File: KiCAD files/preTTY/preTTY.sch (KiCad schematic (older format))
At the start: 27 parts, among them J1 Power Bus, J2 Signal Buss, J3 TTL/RS232, J4 PORT0 TTL, J5 PORT1 TTL/RS232, J6 DB9, U1 74LS07, U2 ATmega328P-PU, U3 MAX232, Y1 16MHz

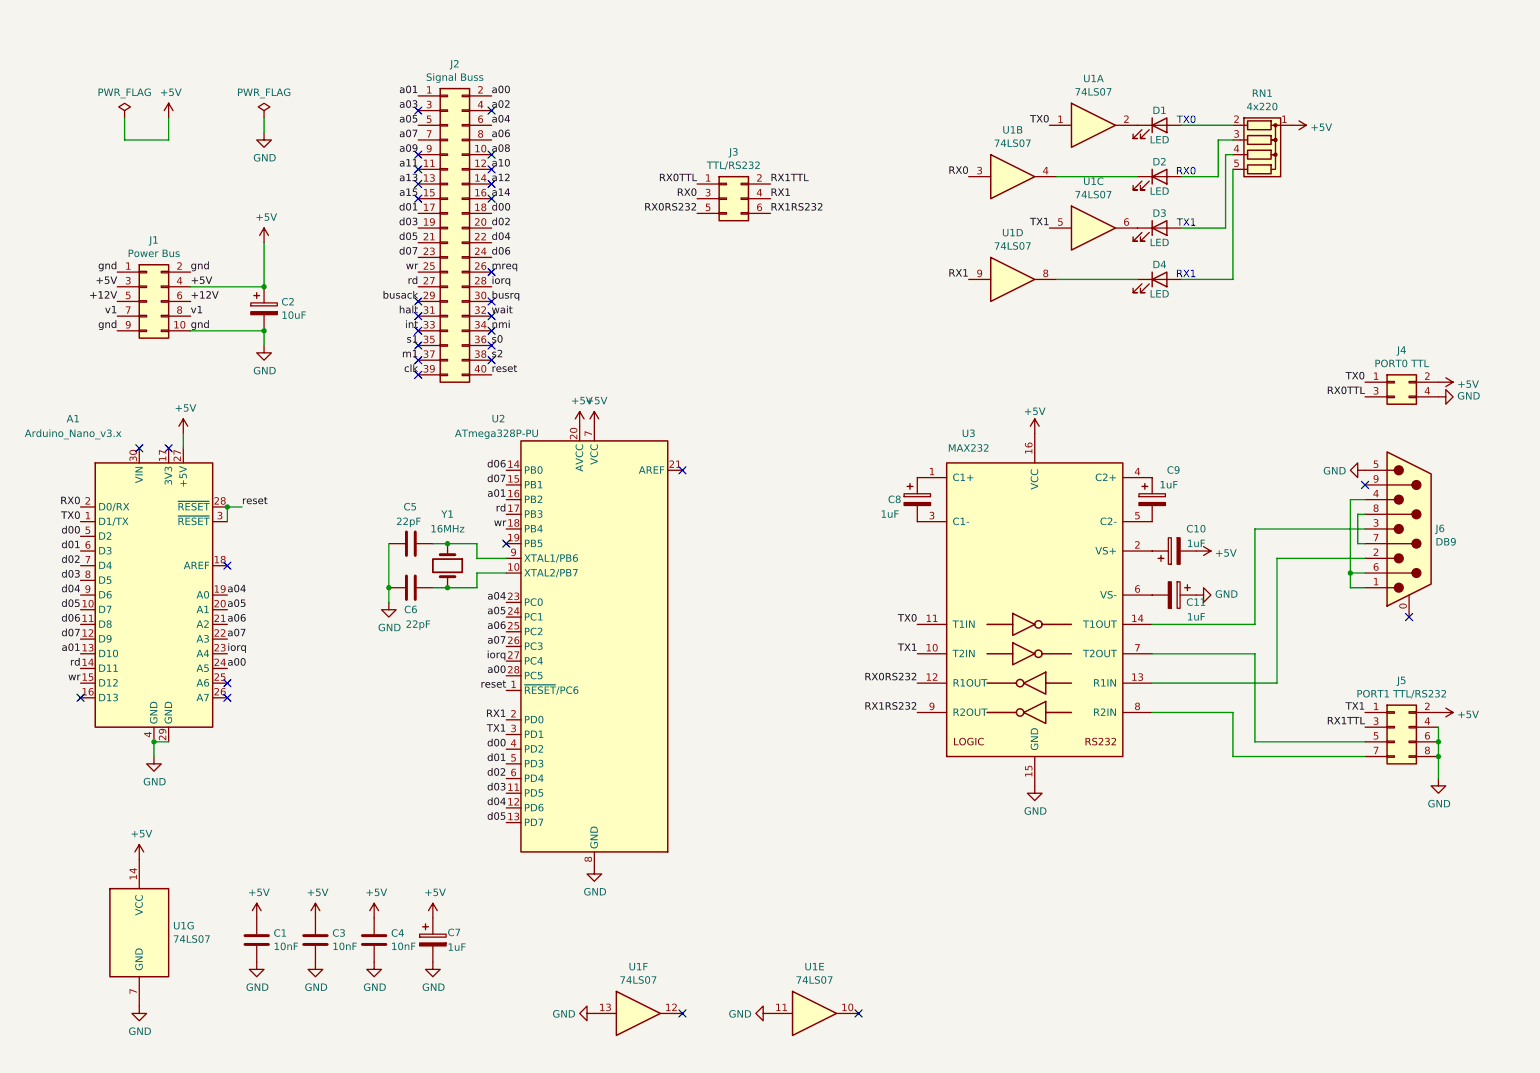
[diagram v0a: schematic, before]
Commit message: office
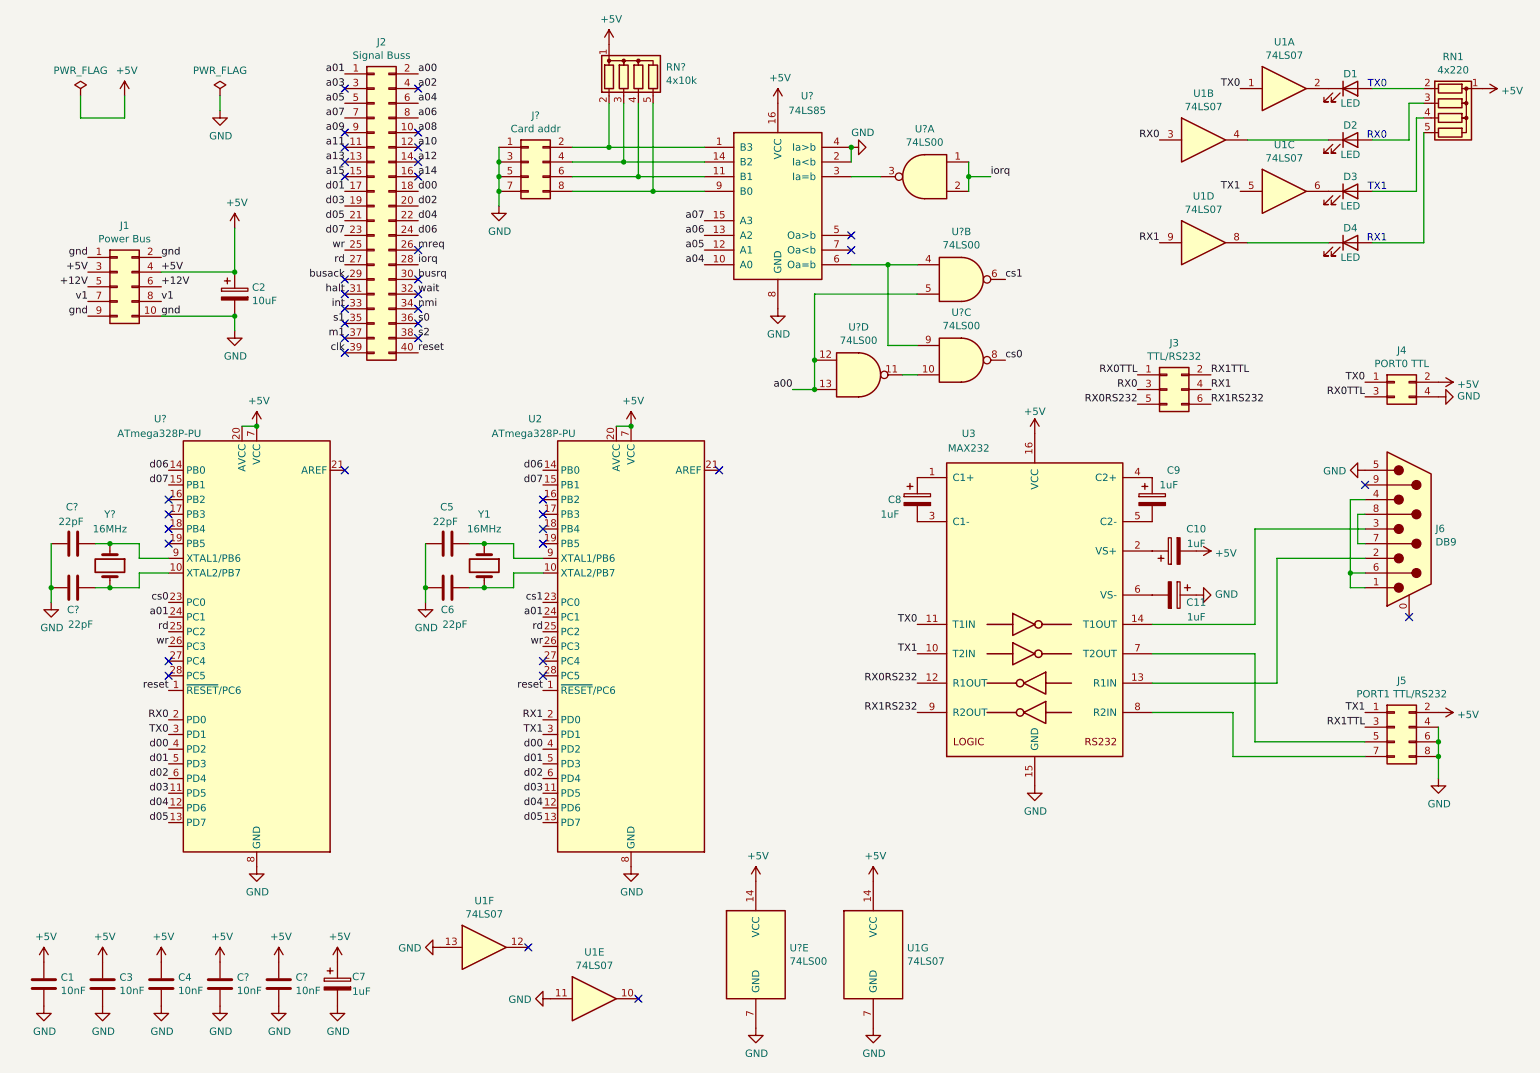
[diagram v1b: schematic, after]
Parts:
- removed A1: Arduino_Nano_v3.x, Module:Arduino_Nano, symbol preTTY-rescue:Arduino_Nano_v3.x-MCU_Module-USARTv2-rescue
- added C? (x2): 22pF, symbol Device:C
- added C? (x2): 10nF, symbol Device:C
- added J?: Card addr, symbol Connector_Generic:Conn_02x04_Odd_Even
- added RN?: 4x10k, Resistor_THT:R_Array_SIP5, symbol Device:R_Network04
- added U?: ATmega328P-PU, Package_DIP:DIP-28_W7.62mm, symbol preTTY-rescue:ATmega328P-PU-MCU_Microchip_ATmega
- added U?: 74LS85, symbol 74xx:74LS85
- added U? (x5): 74LS00, symbol 74xx:74LS00
- added Y?: 16MHz, symbol Device:Crystal
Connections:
- net +5V: now also C?.1, C?.1, RN?.1 (common), U?.14 (VCC), U?.16 (VCC), U?.20 (AVCC), U?.7 (VCC)
- net GND: now also C?.2, C?.2, C?.2, C?.2, J?.1 (Pin_1), J?.3 (Pin_3), J?.5 (Pin_5), J?.7 (Pin_7), U?.2 (Ia<b), U?.22 (GND), U?.4 (Ia>b), U?.7 (GND), U?.8 (GND), U?.8 (GND)
- net RX0: now also U?.2 (PD0)
- net TX0: now also U?.3 (PD1)
- net a00: now also U?.12, U?.13, U?.5; no longer U2.28 (PC5)
- net a01: now also U2.24 (PC1), U?.24 (PC1); no longer U2.16 (PB2)
- net a04: now also U?.10 (A0); no longer U2.23 (PC0)
- net a05: now also U?.12 (A1); no longer U2.24 (PC1)
- net a06: now also U?.13 (A2); no longer U2.25 (PC2)
- net a07: now also U?.15 (A3); no longer U2.26 (PC3)
- net d00: now also U?.4 (PD2)
- net d01: now also U?.5 (PD3)
- net d02: now also U?.6 (PD4)
- net d03: now also U?.11 (PD5)
- net d04: now also U?.12 (PD6)
- net d05: now also U?.13 (PD7)
- net d06: now also U?.14 (PB0)
- net d07: now also U?.15 (PB1)
- net iorq: now also U?.1, U?.2; no longer U2.27 (PC4)
- net rd: now also U2.25 (PC2), U?.25 (PC2); no longer U2.17 (PB3)
- net reset: now also U?.1 (~RESET~/PC6)
- net wr: now also U2.26 (PC3), U?.26 (PC3); no longer U2.18 (PB4)
- new net: C?.1, U?.10 (XTAL2/PB7), Y?.2
- new net: C?.1, U?.9 (XTAL1/PB6), Y?.1
- new net: J?.2 (Pin_2), RN?.2 (R1), U?.1 (B3)
- new net: J?.6 (Pin_6), RN?.4 (R3), U?.11 (B1)
- new net: J?.4 (Pin_4), RN?.3 (R2), U?.14 (B2)
- new net: U?.3, U?.3 (Ia=b)
- new net: U?.4, U?.6 (Oa=b), U?.9
- new net: J?.8 (Pin_8), RN?.5 (R4), U?.9 (B0)
- new net: U?.10, U?.11
- new net cs0: U?.23 (PC0), U?.8
- new net cs1: U2.23 (PC0), U?.6
- no-connect marks 34 -> 42
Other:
- moved on the sheet: C1, C2, C3, C4, C5, C6, C7, D1, D2, D3, D4, J1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
